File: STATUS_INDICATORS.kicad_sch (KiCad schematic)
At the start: 8 parts

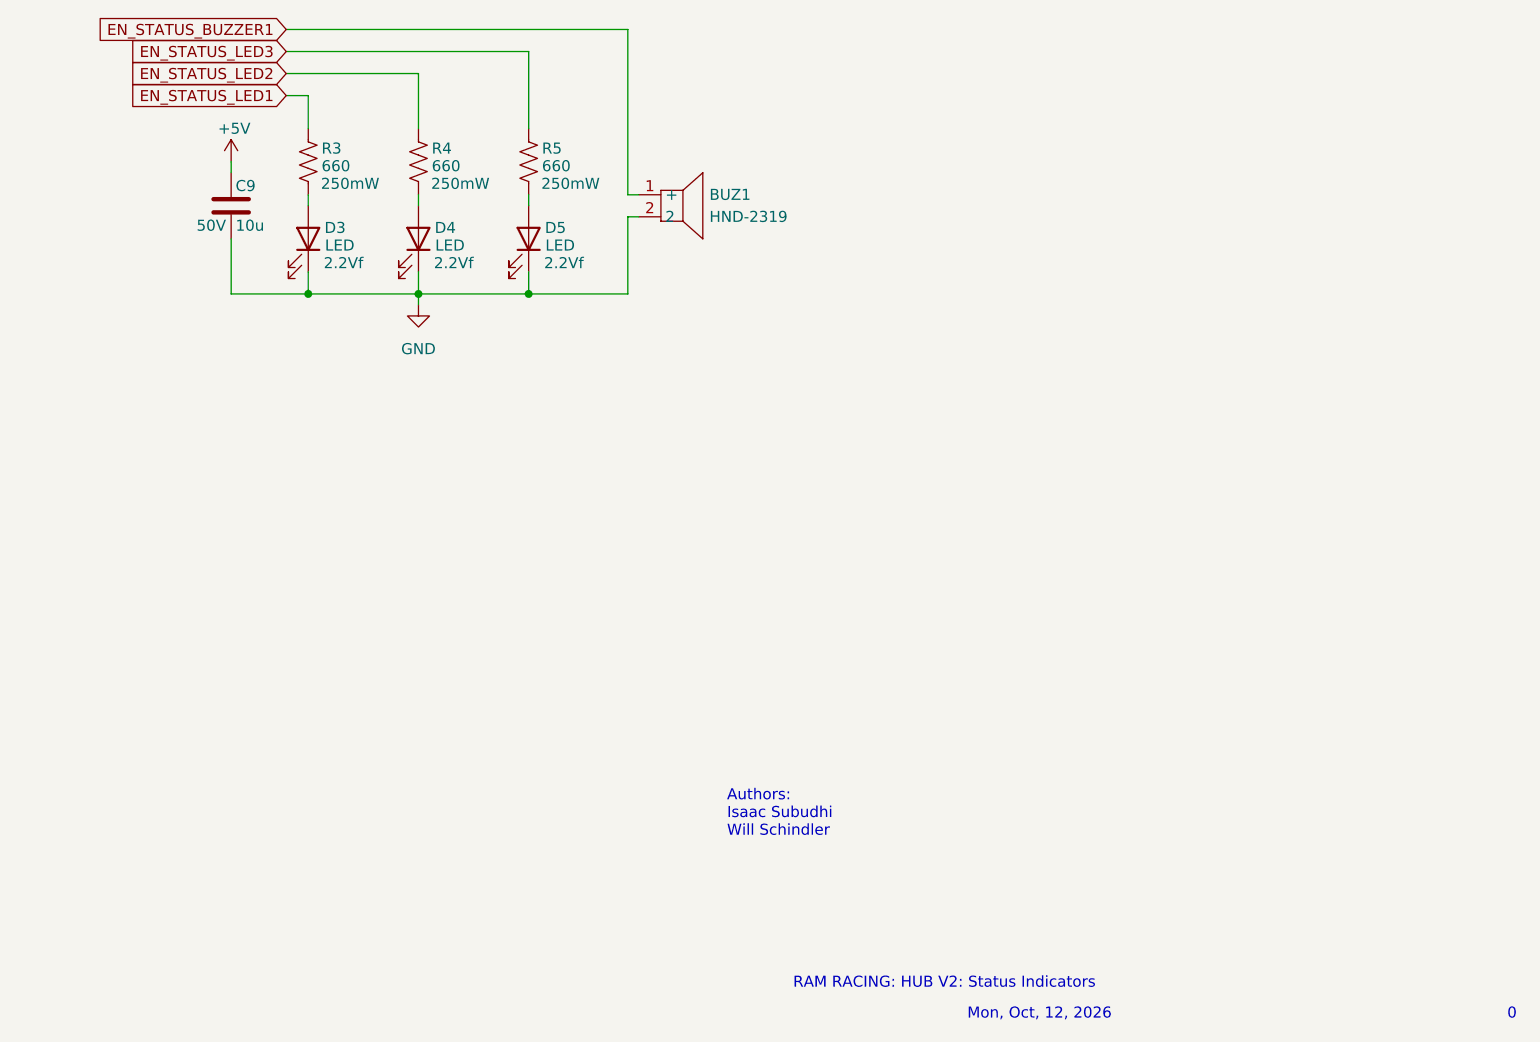
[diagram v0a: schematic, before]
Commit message: Mapping for M130, cleanup on all sheets, layout start
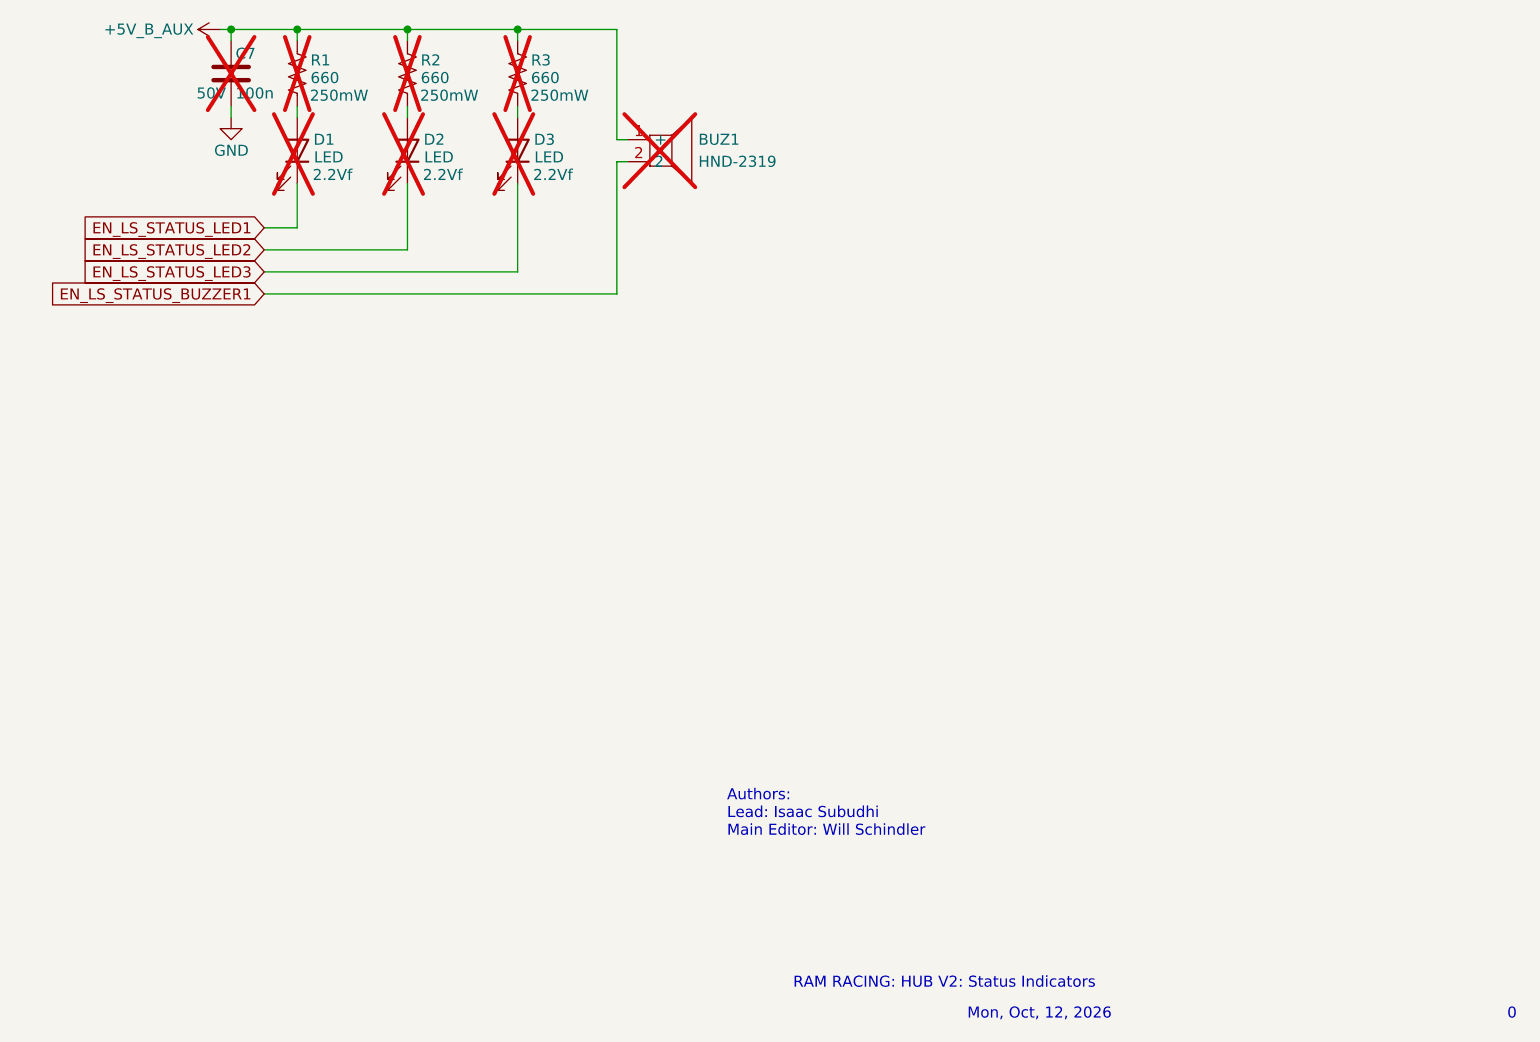
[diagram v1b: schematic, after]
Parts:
- removed C9: 10u, EasyEDA:CAP-TH_L5.5-W3.8-P5.08-D0.5, symbol Device:C
- added C7: 100n, EasyEDA:CAP-TH_L5.0-W2.5-P5.00-D1.0, symbol Device:C
- BUZ1: now not fitted
- D1: renamed from D3; now not fitted
- D2: renamed from D4; now not fitted
- D3: renamed from D5; now not fitted
- R1: renamed from R3; now not fitted
- R2: renamed from R4; now not fitted
- R3: renamed from R5; now not fitted
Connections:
- net EN_STATUS_LED1 is gone; now on net +5V_B_AUX: R1.1
- net EN_STATUS_LED2 is gone; now on net +5V_B_AUX: R2.1
- net EN_STATUS_LED3 is gone; now on net +5V_B_AUX: R3.1
- net GND: now also C7.2; no longer BUZ1.2, D1.1 (K), D2.1 (K), D3.1 (K)
- net EN_STATUS_BUZZER1 renamed +5V_B_AUX
- net +5V_B_AUX: now also C7.1
- new net EN_LS_STATUS_BUZZER1: BUZ1.2
- new net EN_LS_STATUS_LED1: D1.1 (K)
- new net EN_LS_STATUS_LED2: D2.1 (K)
- new net EN_LS_STATUS_LED3: D3.1 (K)
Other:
- note added: "Authors: Lead: Isaac Subudhi Main Editor: Will Schindler"
- note removed: "Authors: Isaac Subudhi Will Schindler"
